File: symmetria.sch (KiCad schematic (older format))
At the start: 97 parts, among them J2 USB_C_Receptacle_USB2.0, SW1 SW_Push, U1 SRV05-4, U2 ATmega32U4-AU, Y1 16MHz

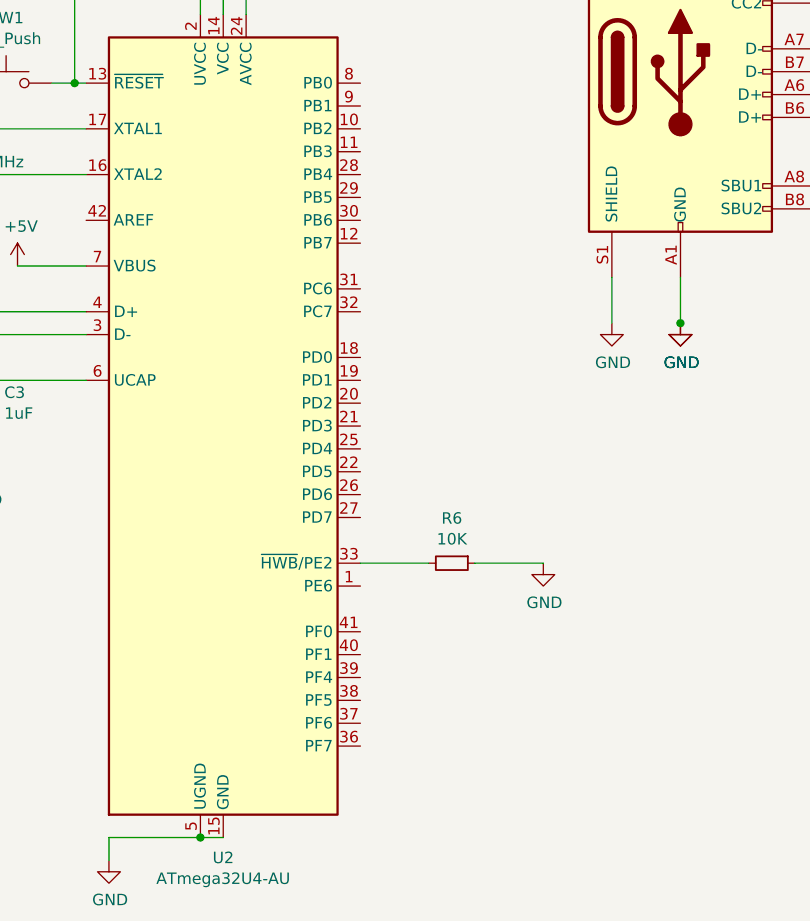
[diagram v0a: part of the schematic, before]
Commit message: PCB Laid out
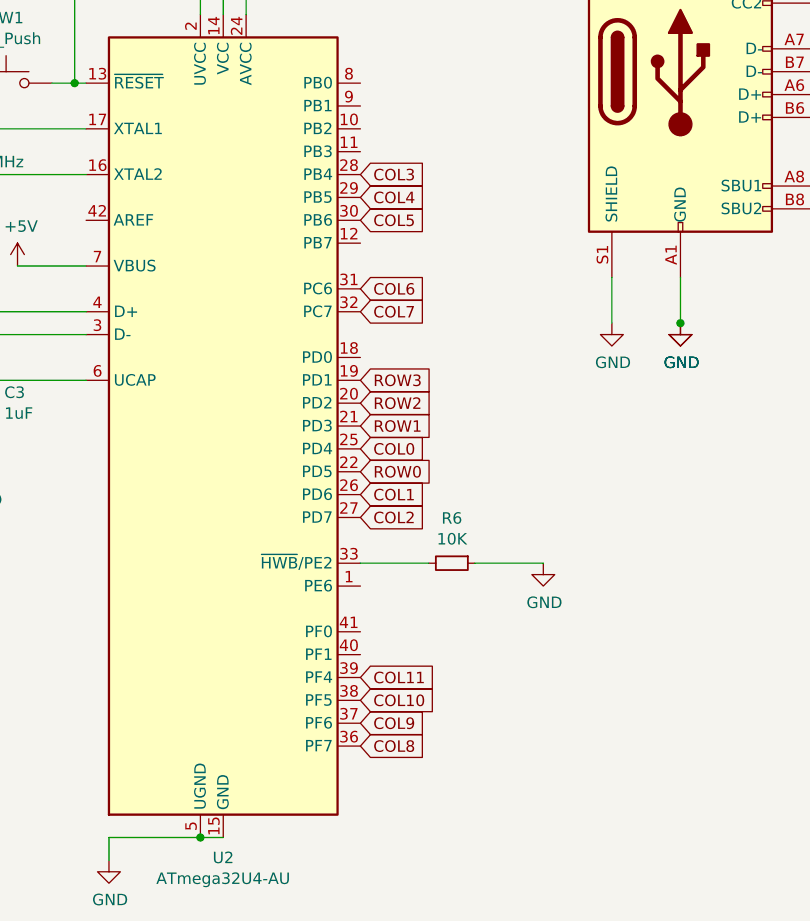
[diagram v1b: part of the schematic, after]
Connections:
- net COL0: now also U2.25 (PD4)
- net COL1: now also U2.26 (PD6)
- net COL10: now also U2.38 (PF5)
- net COL11: now also U2.39 (PF4)
- net COL2: now also U2.27 (PD7)
- net COL3: now also U2.28 (PB4)
- net COL4: now also U2.29 (PB5)
- net COL5: now also U2.30 (PB6)
- net COL6: now also U2.31 (PC6)
- net COL7: now also U2.32 (PC7)
- net COL8: now also U2.36 (PF7)
- net COL9: now also U2.37 (PF6)
- net ROW0: now also U2.22 (PD5)
- net ROW1: now also U2.21 (PD3)
- net ROW2: now also U2.20 (PD2)
- net ROW3: now reaches U2.19 (PD1)
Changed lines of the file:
@@
 Wire Wire Line
 	8150 1200 8650 1200
+Text GLabel 6050 4200 2    50   Input ~ 0
+ROW0
+Text GLabel 6050 4000 2    50   Input ~ 0
+ROW1
+Text GLabel 6050 3900 2    50   Input ~ 0
+ROW2
+Text GLabel 6050 3800 2    50   Input ~ 0
+ROW3
+Text GLabel 6050 5100 2    50   Input ~ 0
+COL11
+Text GLabel 6050 5200 2    50   Input ~ 0
+COL10
+Text GLabel 6050 5300 2    50   Input ~ 0
+COL9
+Text GLabel 6050 5400 2    50   Input ~ 0
+COL8
+Text GLabel 6050 3500 2    50   Input ~ 0
+COL7
+Text GLabel 6050 3400 2    50   Input ~ 0
+COL6
+Text GLabel 6050 3100 2    50   Input ~ 0
+COL5
+Text GLabel 6050 3000 2    50   Input ~ 0
+COL4
+Text GLabel 6050 2900 2    50   Input ~ 0
+COL3
+Text GLabel 6050 4400 2    50   Input ~ 0
+COL2
+Text GLabel 6050 4300 2    50   Input ~ 0
+COL1
+Text GLabel 6050 4100 2    50   Input ~ 0
+COL0
 $EndSCHEMATC

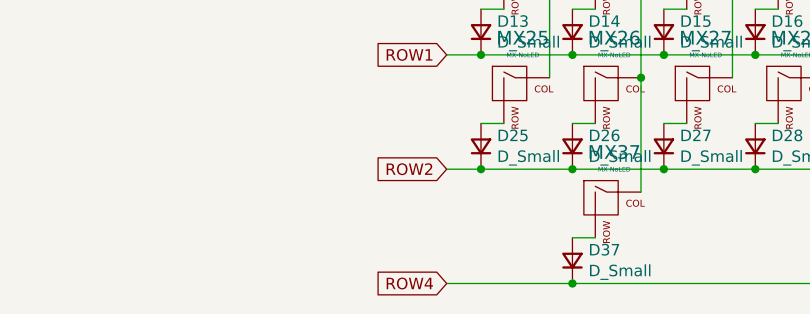
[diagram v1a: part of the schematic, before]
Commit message: Switch Tracing Complete
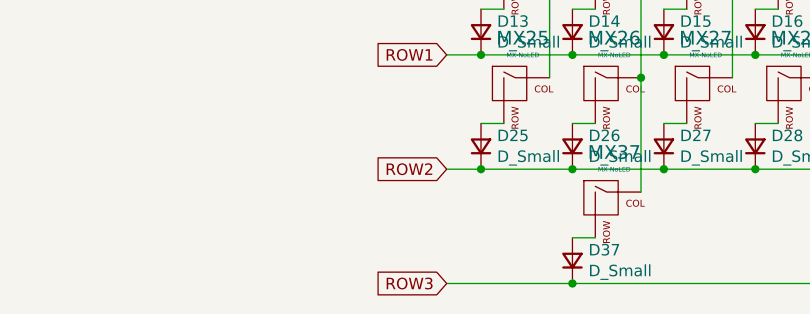
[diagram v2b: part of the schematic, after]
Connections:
- net ROW4 is gone; now on net ROW3: D37.1 (K), D38.1 (K), D39.1 (K)
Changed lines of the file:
@@
 ROW2
 Text GLabel 13100 6400 0    50   Input ~ 0
-ROW4
+ROW3
 Wire Wire Line
 	13100 6400 13650 6400
